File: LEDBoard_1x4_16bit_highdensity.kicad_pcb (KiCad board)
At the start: 2 copper layers, 12.3 x 7 mm, 10 parts, among them J1 signal_in, J2 signal_out, J3 power, U1 TLC5971PWP

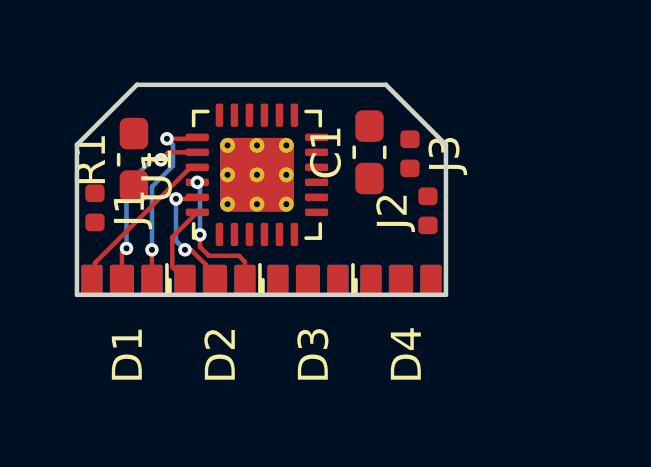
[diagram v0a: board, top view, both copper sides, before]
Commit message: partly routed
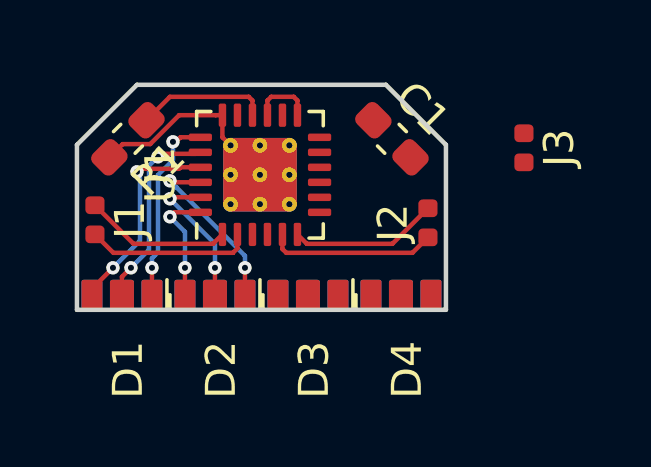
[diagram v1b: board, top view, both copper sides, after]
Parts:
- moved J3 3.81 mm to (114.9, 102.1)
- moved C1 0.87 mm to (110.5, 101.8), turned to 315 degrees
- moved R1 0.73 mm to (101.7, 101.8), turned to 225 degrees
- moved D1 0.50 mm to (101.5, 107.5)
- moved D2 0.50 mm to (104.6, 107.5)
- moved D3 0.50 mm to (107.7, 107.5)
- moved D4 0.50 mm to (110.8, 107.5)
- moved J1 0.40 mm to (100.6, 104.5)
- moved J2 0.40 mm to (111.7, 104.6)
- moved U1 0.10 mm to (106.1, 103.0)
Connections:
- net Net-(R1-Pad1) renamed /IREF
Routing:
- net /clock_out: track 0.00 -> 5.60 mm
- net /clock_in: track 0.00 -> 5.53 mm
- net GND: track 0.00 -> 5.47 mm
- net /data_out: track 0.00 -> 4.97 mm
- net /data_in: track 0.00 -> 4.91 mm
- net /IREF: track 0.00 -> 4.39 mm
- net VCC: track 0.00 -> 2.08 mm
- net /led_0_b: track 5.34 -> 7.05 mm, vias 0 -> 2
- net /led_1_r: track 4.49 -> 5.87 mm
- net /led_1_b: track 2.77 -> 3.88 mm, vias 0 -> 2
- net /led_1_g: track 4.08 -> 4.85 mm
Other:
- board size 12.3 x 7 mm -> 12.3 x 7.5 mm
